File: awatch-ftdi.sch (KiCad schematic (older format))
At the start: 42 parts

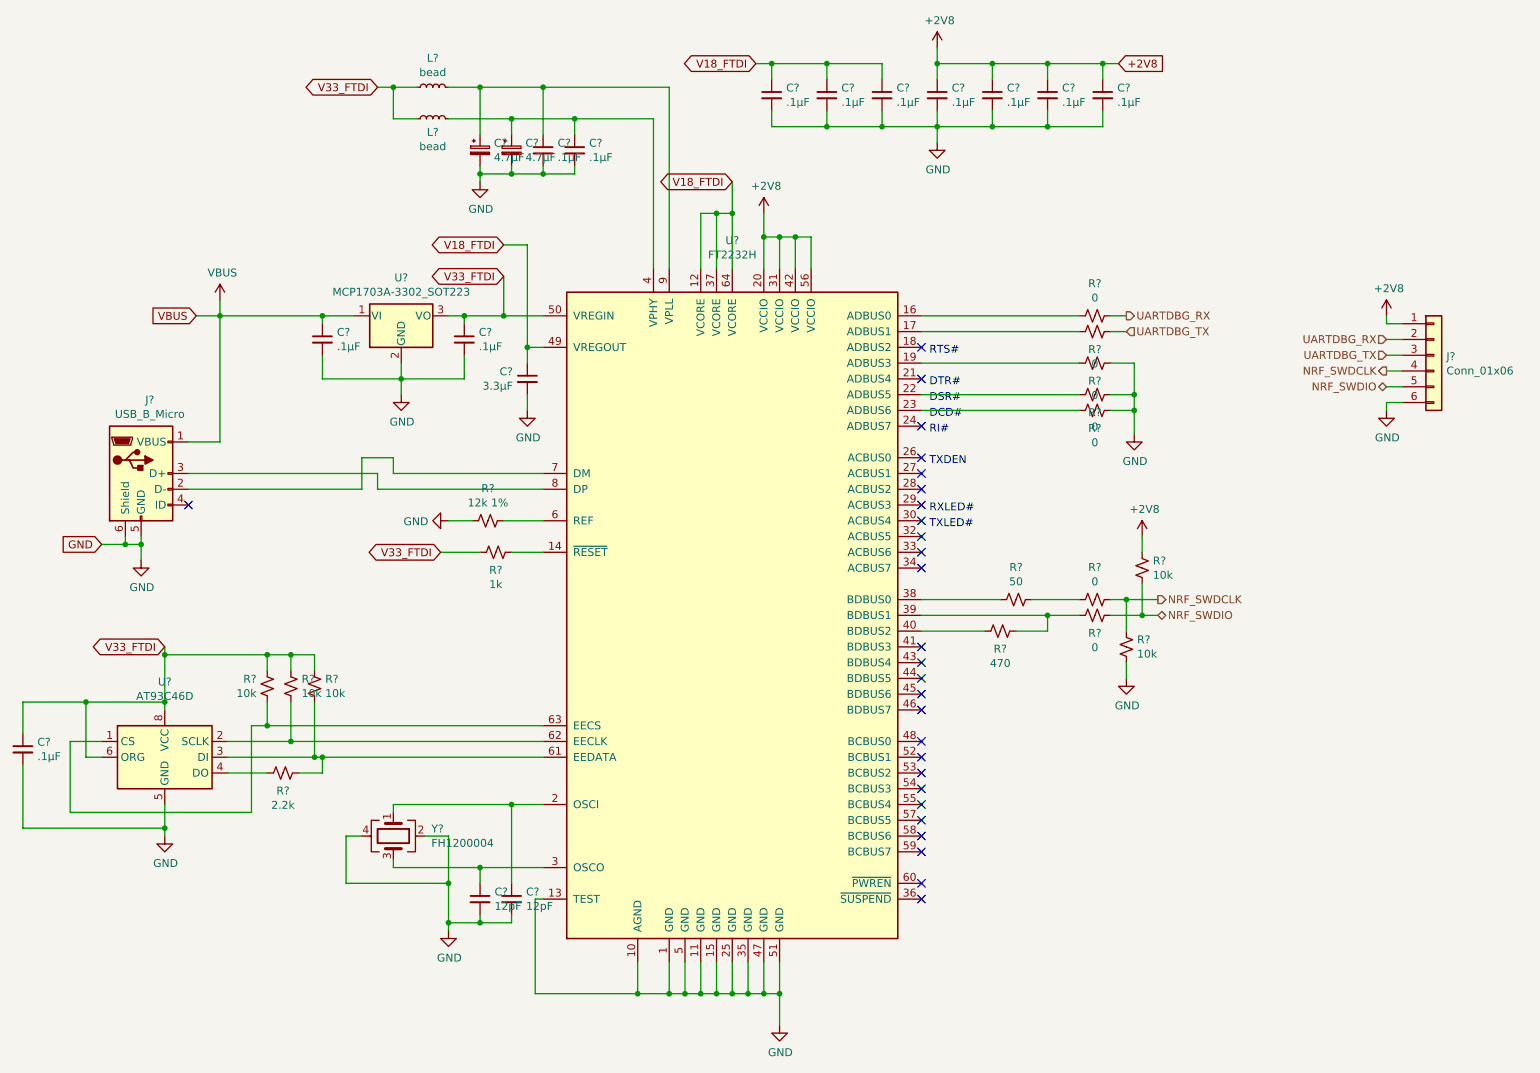
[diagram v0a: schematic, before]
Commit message: annotate all
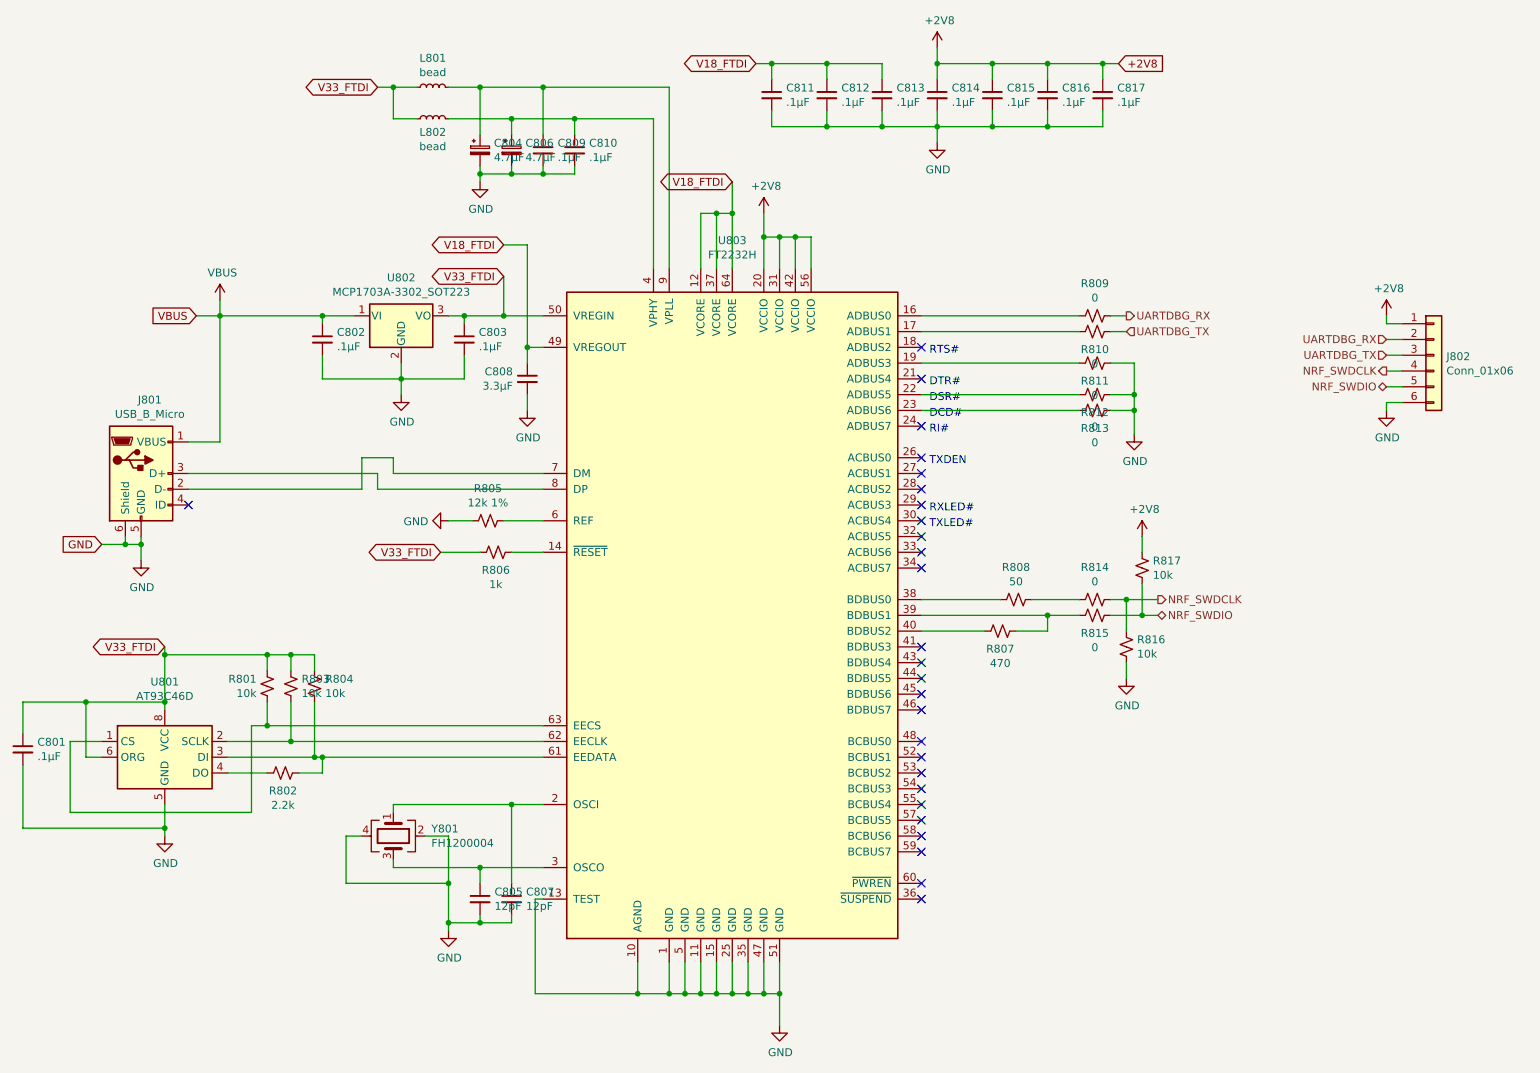
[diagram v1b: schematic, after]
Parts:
- gave numbers to parts that had none: 42
